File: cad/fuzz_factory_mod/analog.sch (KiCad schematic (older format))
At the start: 8 parts

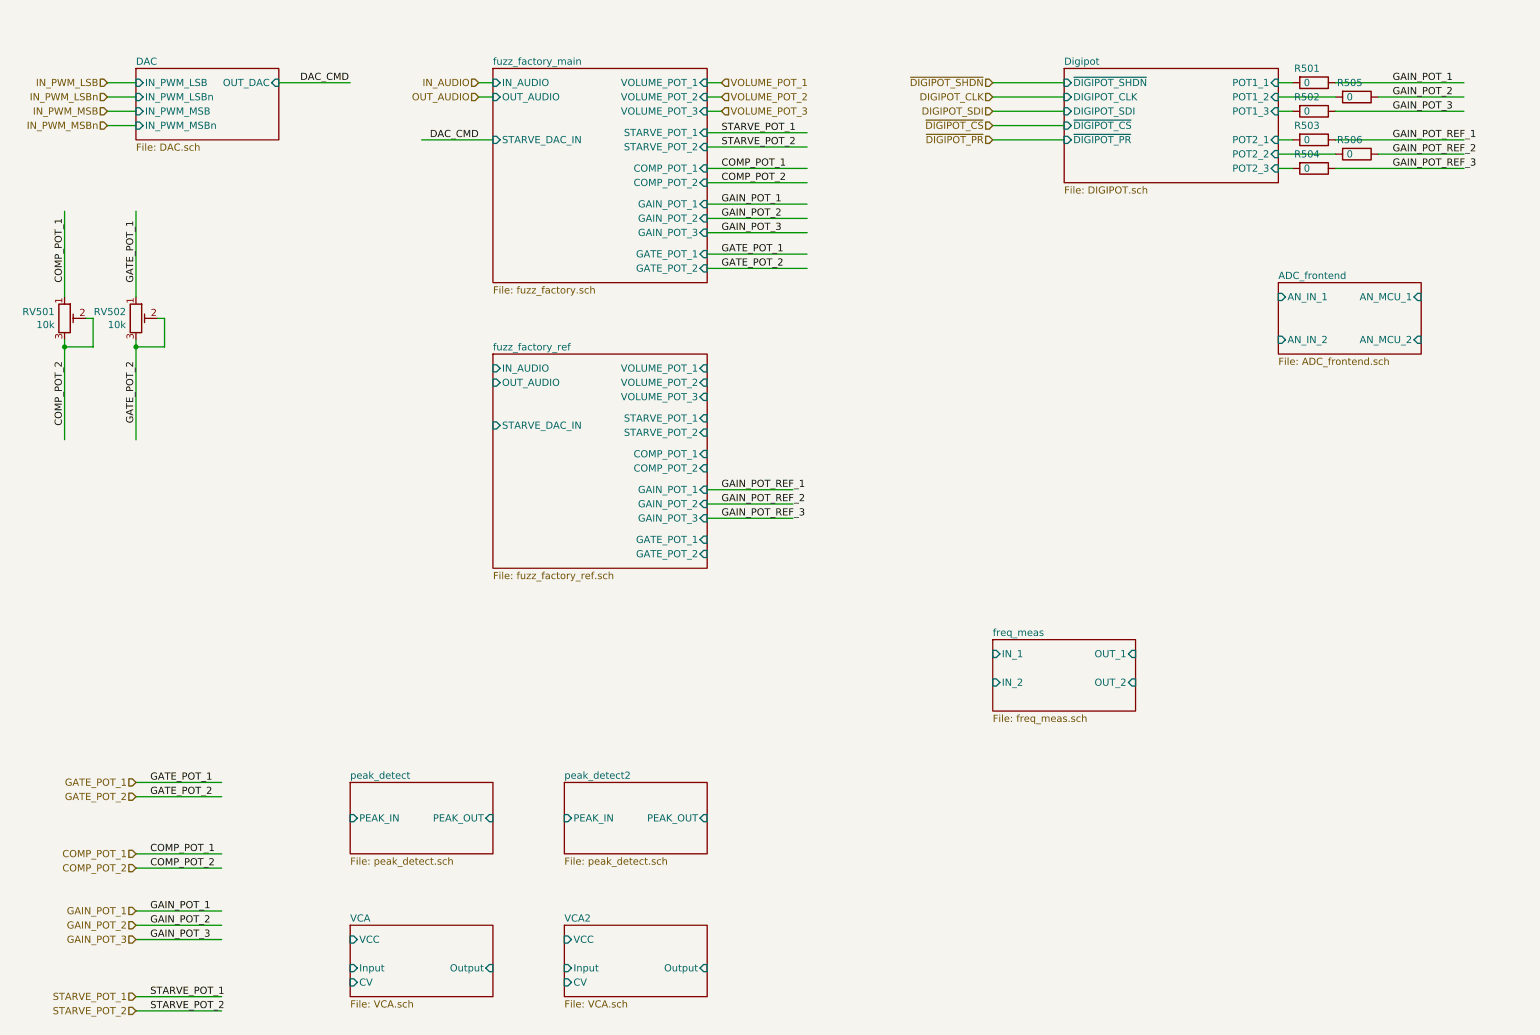
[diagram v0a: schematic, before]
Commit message: Continued schematic.
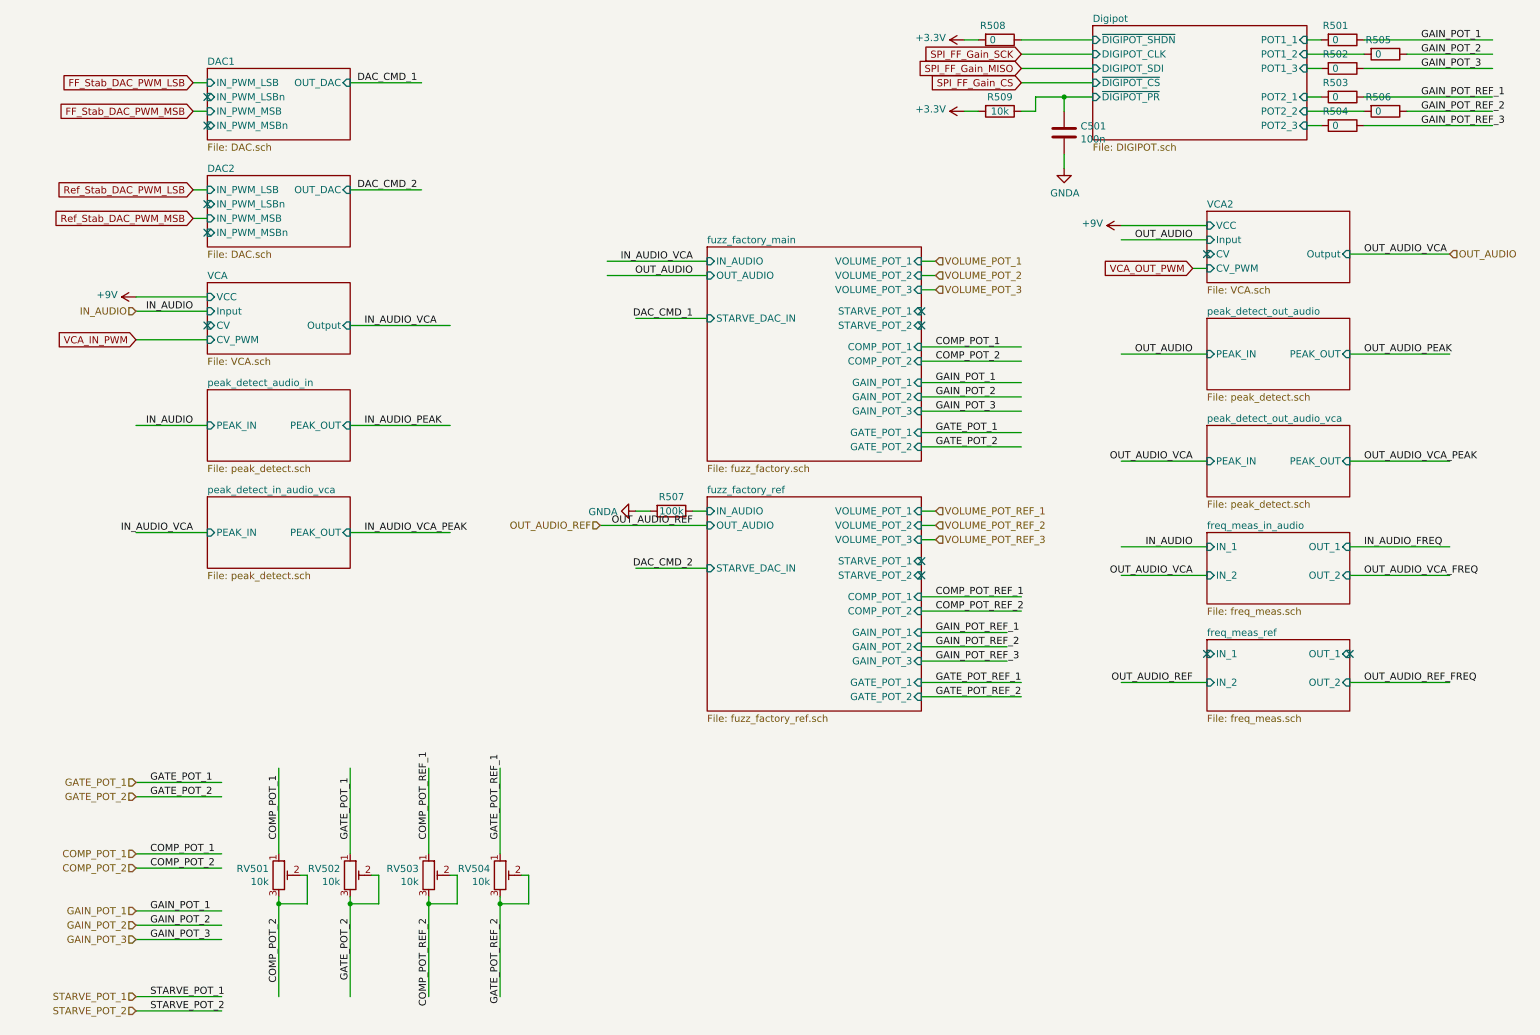
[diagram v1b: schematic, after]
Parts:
- added C501: 100n, Capacitors_SMD:C_0603, symbol Device:C
- added R507: 100k, Resistors_SMD:R_0603, symbol Device:R
- added R508: 0, Resistors_SMD:R_0603, symbol Device:R
- added R509: 10k, Resistors_SMD:R_0603, symbol Device:R
- added RV503, RV504: 10k, Potentiometers:Potentiometer_Trimmer_Bourns_3266X, symbol Device:R_POT_TRIM
- RV501, RV502: footprint (none) -> Potentiometers:Potentiometer_Trimmer_Bourns_3266X
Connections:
- net labels added: +3.3V, +9V, COMP_POT_REF_1, COMP_POT_REF_2, DAC_CMD_1, DAC_CMD_2, FF_Stab_DAC_PWM_LSB, FF_Stab_DAC_PWM_MSB, GATE_POT_REF_1, GATE_POT_REF_2, GNDA, IN_AUDIO_FREQ, IN_AUDIO_PEAK, IN_AUDIO_VCA, IN_AUDIO_VCA_PEAK, OUT_AUDIO_PEAK, OUT_AUDIO_REF, OUT_AUDIO_REF_FREQ, OUT_AUDIO_VCA, OUT_AUDIO_VCA_FREQ, OUT_AUDIO_VCA_PEAK, Ref_Stab_DAC_PWM_LSB, Ref_Stab_DAC_PWM_MSB, SPI_FF_Gain_CS, SPI_FF_Gain_MISO, SPI_FF_Gain_SCK, VCA_IN_PWM, VCA_OUT_PWM, VOLUME_POT_REF_1, VOLUME_POT_REF_2, VOLUME_POT_REF_3
- net labels removed: DAC_CMD, DIGIPOT_CLK, DIGIPOT_SDI, IN_PWM_LSB, IN_PWM_LSBn, IN_PWM_MSB, IN_PWM_MSBn, ~DIGIPOT_CS, ~DIGIPOT_PR, ~DIGIPOT_SHDN
- wire segments 61 -> 112
- no-connect marks 0 -> 12
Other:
- moved on the sheet: R501, R502, R503, R504, R505, R506, RV501, RV502
